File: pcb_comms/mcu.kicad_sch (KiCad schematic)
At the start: 22 parts, among them U2 STM32WLE5CCU6, Y3 32MHz

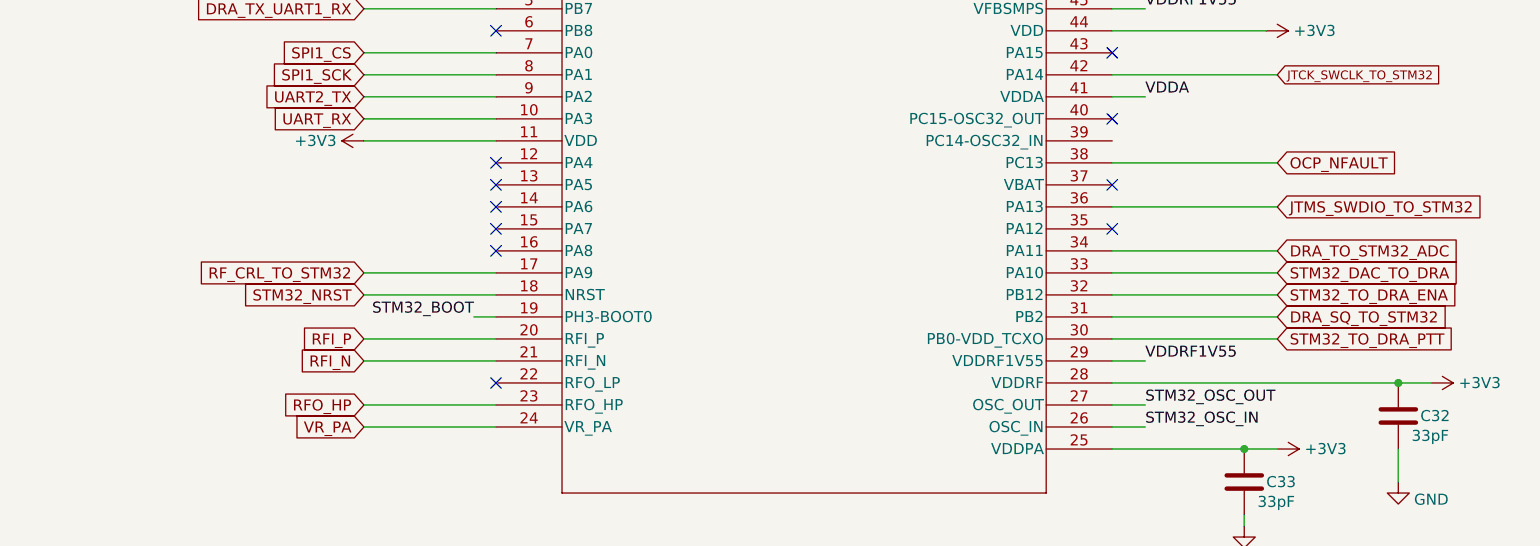
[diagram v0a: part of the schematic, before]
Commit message: PCB v2
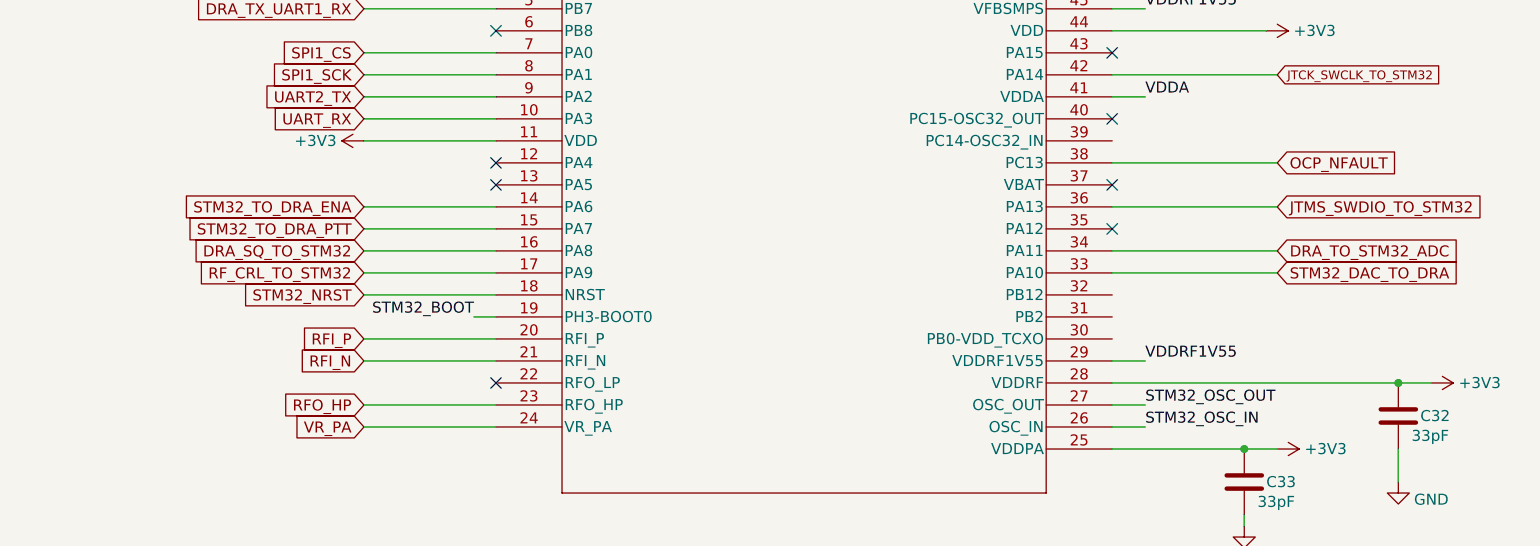
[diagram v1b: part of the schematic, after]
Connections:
- net DRA_SQ_TO_STM32: now also U2.16 (PA8); no longer U2.31 (PB2)
- net STM32_TO_DRA_ENA: now also U2.14 (PA6); no longer U2.32 (PB12)
- net STM32_TO_DRA_PTT: now also U2.15 (PA7); no longer U2.30 (PB0-VDD_TCXO)
- no-connect marks 11 -> 8
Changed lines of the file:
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@@
-	)
-	(no_connect
-		(at 167.64 132.08)
 	)
 	(no_connect
@@
 	)
 	(no_connect
-		(at 167.64 129.54)
-	)
-	(no_connect
 		(at 167.64 127)
-	)
-	(no_connect
-		(at 167.64 134.62)
 	)
 	(no_connect
@@
 	(wire
 		(pts
+			(xy 152.4 132.08) (xy 167.64 132.08)
+		)
+		(stroke
+			(width 0)
+			(type default)
+		)
+	)
+	(wire
+		(pts
 			(xy 238.76 157.48) (xy 254 157.48)
 		)
@@
 	(wire
 		(pts
-			(xy 238.76 142.24) (xy 257.81 142.24)
-		)
-		(stroke
-			(width 0)
-			(type default)
-		)
-	)
-	(wire
-		(pts
 			(xy 123.19 38.1) (xy 123.19 41.91)
 		)
@@
 	(wire
 		(pts
-			(xy 238.76 144.78) (xy 257.81 144.78)
-		)
-		(stroke
-			(width 0)
-			(type default)
-		)
-	)
-	(wire
-		(pts
 			(xy 25.4 46.99) (xy 25.4 36.83)
 		)
@@
 	(wire
 		(pts
+			(xy 152.4 129.54) (xy 167.64 129.54)
+		)
+		(stroke
+			(width 0)
+			(type default)
+		)
+	)
+	(wire
+		(pts
 			(xy 238.76 137.16) (xy 257.81 137.16)
 		)
@@
 	(wire
 		(pts
-			(xy 238.76 139.7) (xy 257.81 139.7)
-		)
-		(stroke
-			(width 0)
-			(type default)
-		)
-	)
-	(wire
-		(pts
 			(xy 271.78 149.86) (xy 275.59 149.86)
 		)
@@
 		(pts
 			(xy 45.72 161.29) (xy 58.42 161.29)
+		)
+		(stroke
+			(width 0)
+			(type default)
+		)
+	)
+	(wire
+		(pts
+			(xy 152.4 134.62) (xy 167.64 134.62)
 		)
 		(stroke
@@
 	(global_label "DRA_SQ_TO_STM32"
 		(shape input)
-		(at 257.81 142.24 0)
-		(effects
-			(font
-				(size 1.27 1.27)
-			)
-			(justify left)
-		)
-		(property "Intersheetrefs" "${INTERSHEET_REFS}"
-			(at 279.4822 129.54 0)
-			(effects
-				(font
-					(size 1.27 1.27)
-				)
-				(justify left)
+		(at 152.4 134.62 180)
+		(effects
+			(font
+				(size 1.27 1.27)
+			)
+			(justify right)
+		)
+		(property "Intersheetrefs" "${INTERSHEET_REFS}"
+			(at 130.7278 121.92 0)
+			(effects
+				(font
+					(size 1.27 1.27)
+				)
+				(justify right)
 				(hide yes)
 			)
@@
 	(global_label "STM32_TO_DRA_PTT"
 		(shape input)
-		(at 257.81 144.78 0)
+		(at 152.4 132.08 180)
 		(fields_autoplaced yes)
 		(effects
@@
 				(size 1.27 1.27)
 			)
-			(justify left)
-		)
-		(property "Intersheetrefs" "${INTERSHEET_REFS}"
-			(at 278.8774 144.78 0)
-			(effects
-				(font
-					(size 1.27 1.27)
-				)
-				(justify left)
+			(justify right)
+		)
+		(property "Intersheetrefs" "${INTERSHEET_REFS}"
+			(at 131.3326 132.08 0)
+			(effects
+				(font
+					(size 1.27 1.27)
+				)
+				(justify right)
 				(hide yes)
 			)
@@
 	(global_label "STM32_TO_DRA_ENA"
 		(shape input)
-		(at 257.81 139.7 0)
+		(at 152.4 129.54 180)
 		(fields_autoplaced yes)
 		(effects
@@
 				(size 1.27 1.27)
 			)
-			(justify left)
-		)
-		(property "Intersheetrefs" "${INTERSHEET_REFS}"
-			(at 279.2403 139.7 0)
-			(effects
-				(font
-					(size 1.27 1.27)
-				)
-				(justify left)
-				(hide yes)
-			)
+			(justify right)
+		)
+		(property "Intersheetrefs" "${INTERSHEET_REFS}"
+			(at 130.9697 129.54 0)
+			(effects
+				(font
+					(size 1.27 1.27)
+				)
+				(justify right)
+				(hide yes)
+			)

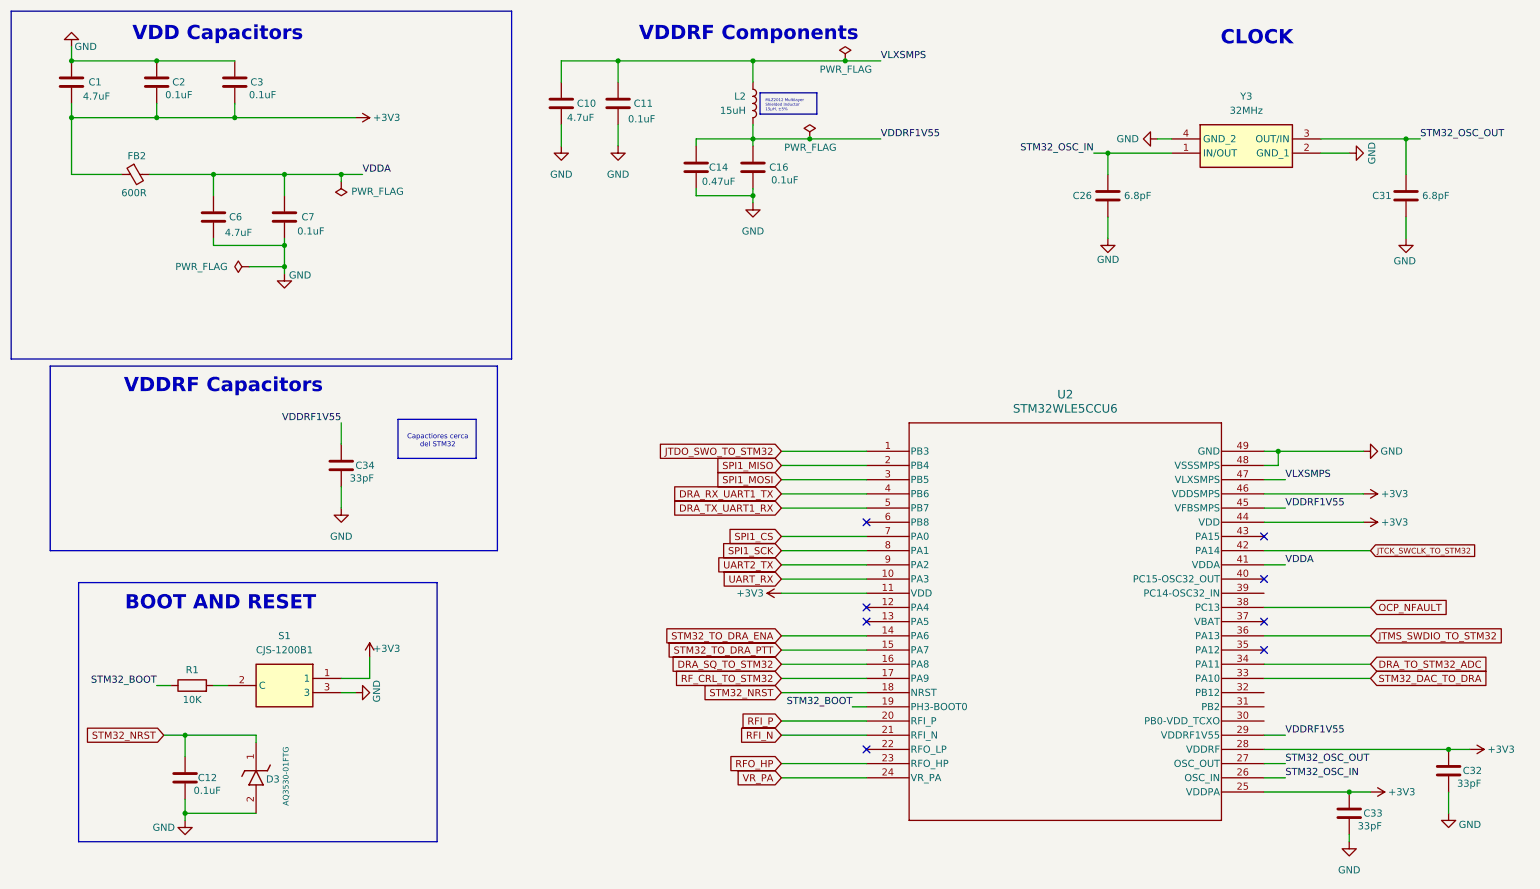
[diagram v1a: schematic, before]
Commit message: PCB v2.1
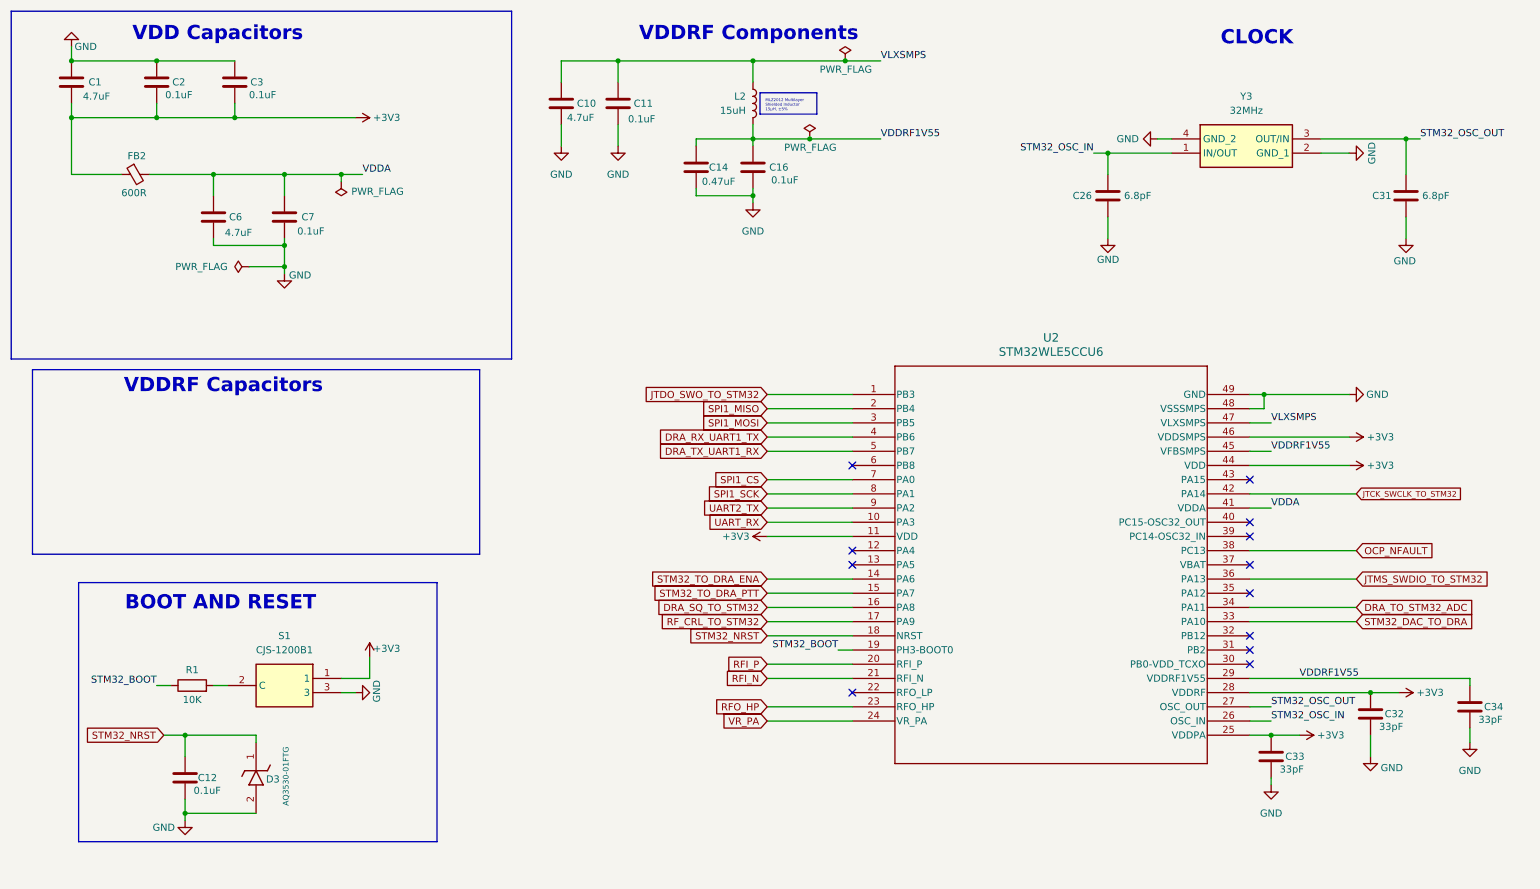
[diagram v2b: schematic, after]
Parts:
- C1, C10, C11, C14, C16, C2, C26, C3, C31, C32, C34, C6, C7: footprint Capacitor_SMD:C_0805_2012Metric_Pad1.18x1.45mm_HandSolder -> Capacitor_SMD:C_0603_1608Metric_Pad1.08x0.95mm_HandSolder
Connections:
- no-connect marks 8 -> 12
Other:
- note removed: "Capactiores cerca del STM32"
- moved on the sheet: C32, C33, C34, U2
